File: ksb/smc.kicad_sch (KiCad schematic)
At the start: 15 parts, among them U4 X850744-001

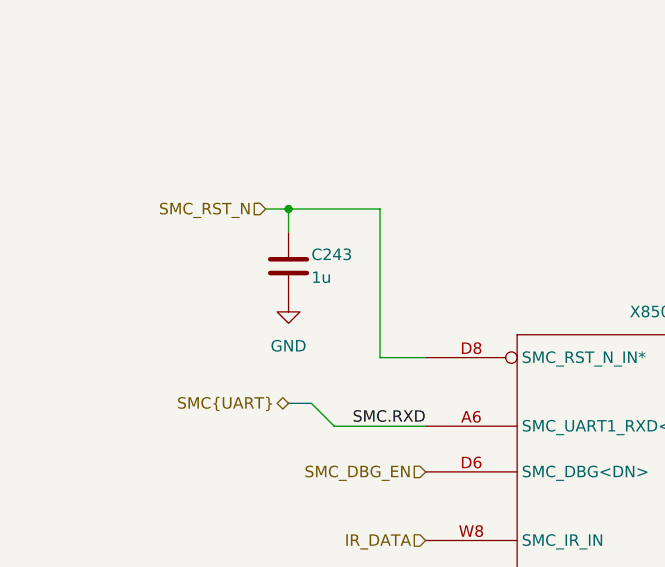
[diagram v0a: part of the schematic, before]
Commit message: Cleanup & Debug I/O
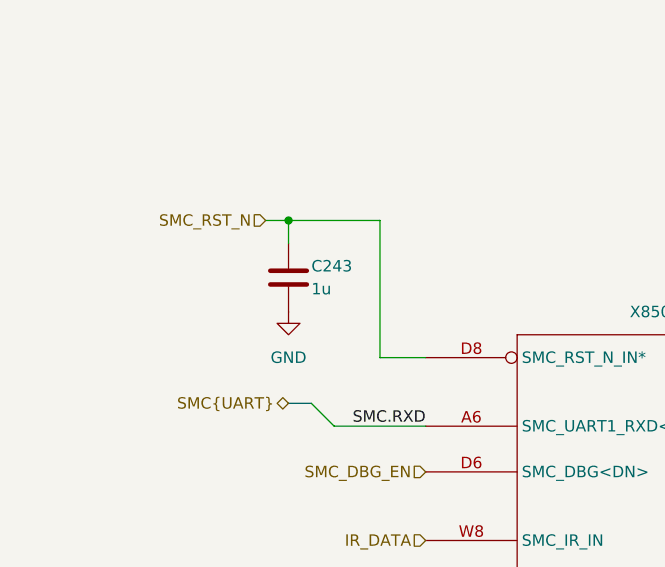
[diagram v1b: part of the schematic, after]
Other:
- moved on the sheet: C243
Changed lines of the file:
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@@
 	)
 	(junction
-		(at 48.26 78.74)
+		(at 48.26 80.01)
 		(diameter 0)
 		(color 0 0 0 0)
@@
 	(wire
 		(pts
-			(xy 45.72 78.74) (xy 48.26 78.74)
+			(xy 45.72 80.01) (xy 48.26 80.01)
 		)
 		(stroke
@@
 	(wire
 		(pts
-			(xy 58.42 78.74) (xy 48.26 78.74)
+			(xy 58.42 80.01) (xy 48.26 80.01)
 		)
 		(stroke
@@
 	(wire
 		(pts
-			(xy 58.42 95.25) (xy 58.42 78.74)
+			(xy 58.42 95.25) (xy 58.42 80.01)
 		)
 		(stroke
@@
 	(wire
 		(pts
-			(xy 48.26 81.28) (xy 48.26 78.74)
+			(xy 48.26 82.55) (xy 48.26 80.01)
 		)
 		(stroke
@@
 	(hierarchical_label "SMC_RST_N"
 		(shape input)
-		(at 45.72 78.74 180)
+		(at 45.72 80.01 180)
 		(effects
 			(font
@@
 	(symbol
 		(lib_id "Device:C")
-		(at 48.26 85.09 0)
+		(at 48.26 86.36 0)
 		(unit 1)
 		(exclude_from_sim no)
@@
 		(dnp no)
 		(property "Reference" "C243"
-			(at 50.8 83.82 0)
+			(at 50.8 85.09 0)
 			(effects
 				(font
@@
 		)
 		(property "Value" "1u"
-			(at 50.8 86.36 0)
+			(at 50.8 87.63 0)
 			(effects
 				(font
@@
 		)
 		(property "Footprint" ""
-			(at 49.2252 88.9 0)
+			(at 49.2252 90.17 0)
 			(effects
 				(font
@@
 		)
 		(property "Datasheet" "~"
-			(at 48.26 85.09 0)
+			(at 48.26 86.36 0)
 			(effects
 				(font
@@
 		)
 		(property "Description" "Unpolarized capacitor"
-			(at 48.26 85.09 0)
+			(at 48.26 86.36 0)
 			(effects
 				(font
@@
 	(symbol
 		(lib_id "power:GND")
-		(at 48.26 88.9 0)
+		(at 48.26 90.17 0)
 		(unit 1)
 		(exclude_from_sim no)
@@
 		(fields_autoplaced yes)
 		(property "Reference" "#PWR0111"
-			(at 48.26 95.25 0)
+			(at 48.26 96.52 0)
 			(effects
 				(font
@@
 		)
 		(property "Value" "GND"
-			(at 48.26 93.98 0)
+			(at 48.26 95.25 0)
 			(effects
 				(font
@@
 		)
 		(property "Footprint" ""
-			(at 48.26 88.9 0)
+			(at 48.26 90.17 0)
 			(effects
 				(font
@@
 		)
 		(property "Datasheet" ""
-			(at 48.26 88.9 0)
+			(at 48.26 90.17 0)
 			(effects
 				(font
@@
 		)
 		(property "Description" "Power symbol creates a global label with name \"GND\" , ground"
-			(at 48.26 88.9 0)
+			(at 48.26 90.17 0)
 			(effects
 				(font
